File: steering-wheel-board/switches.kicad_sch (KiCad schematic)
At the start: 15 parts, among them SW2 SW_SPST, SW3 SW_SPST, SW4 SW_SPST

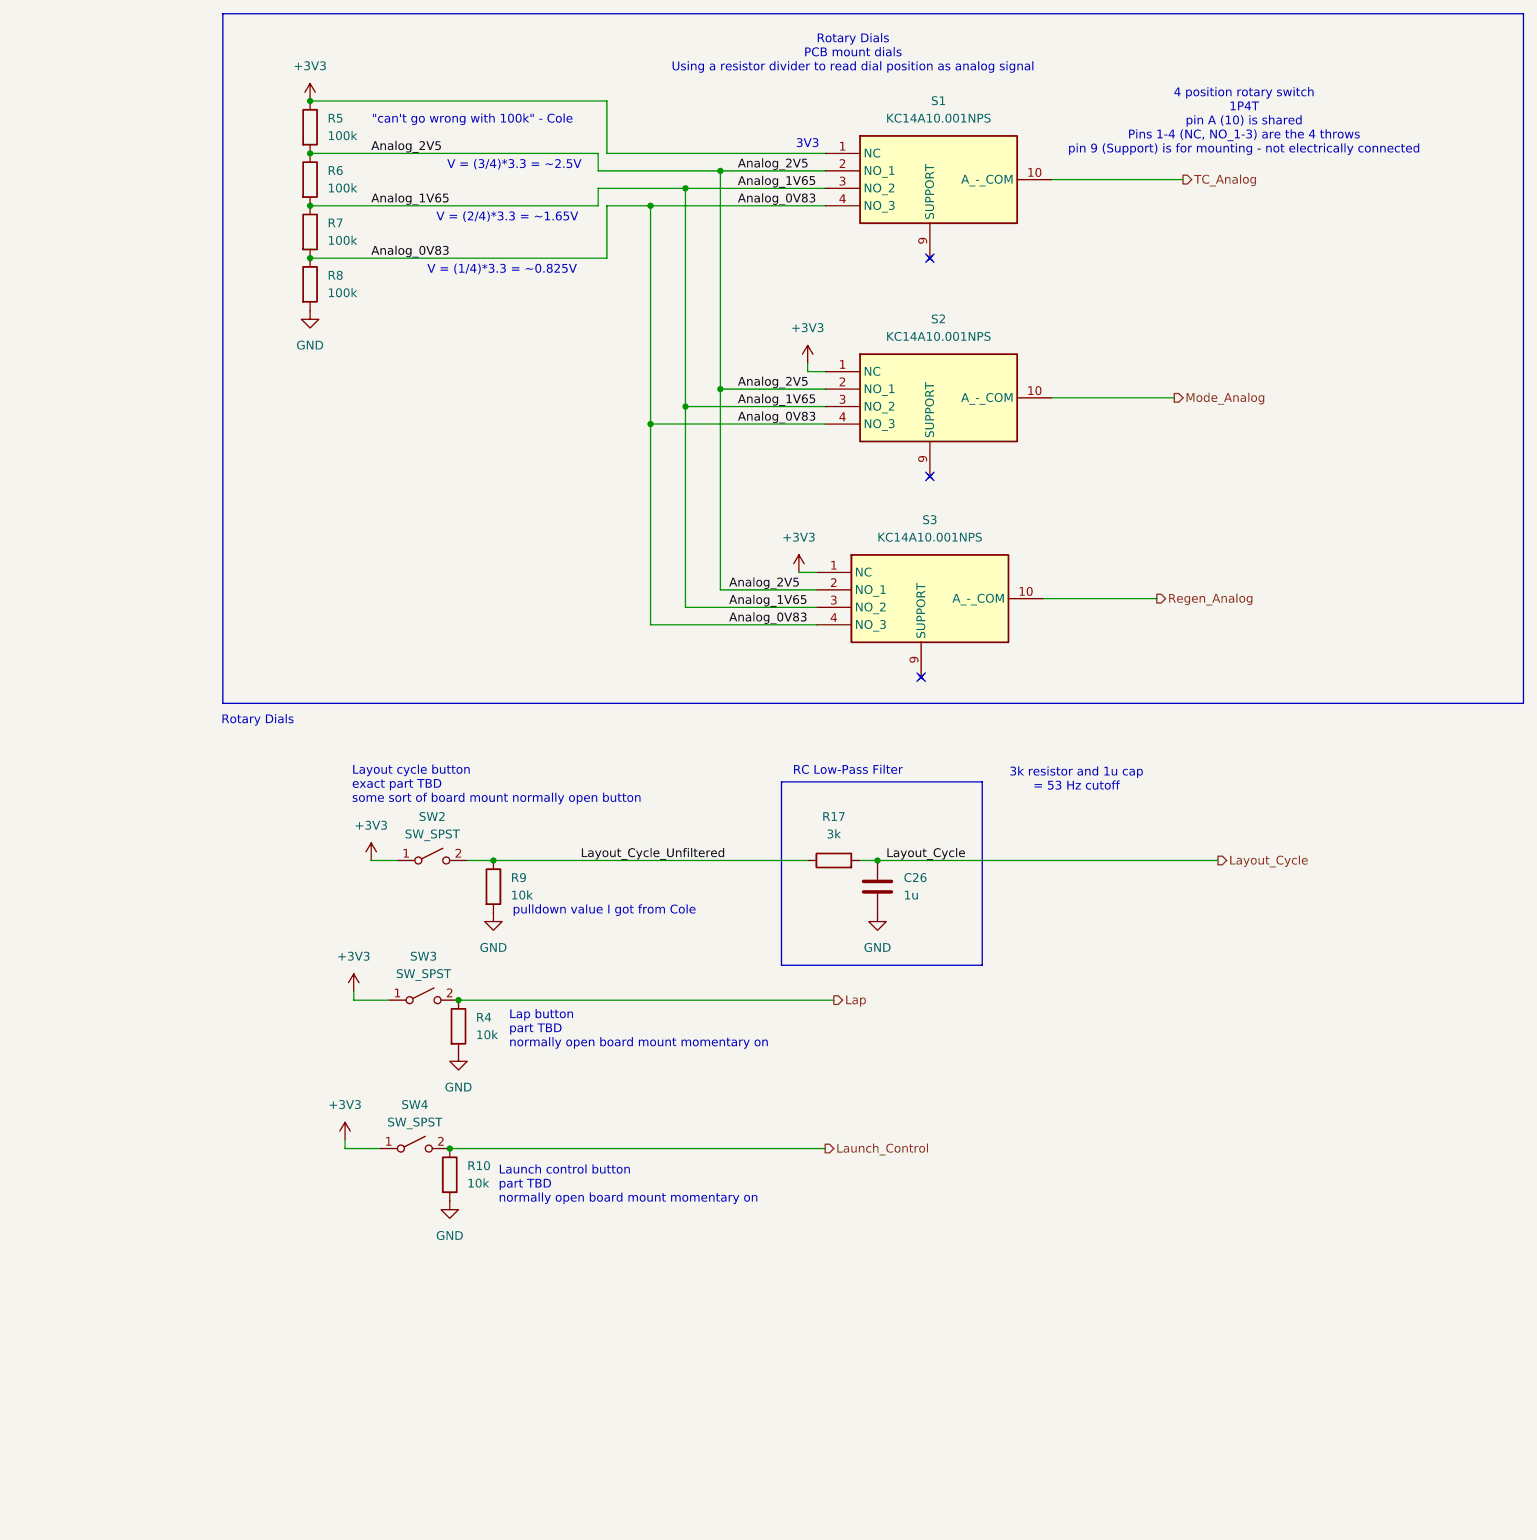
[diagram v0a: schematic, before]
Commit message: formatting changes, updated resistor ladder and CAN termination/aux can jumper
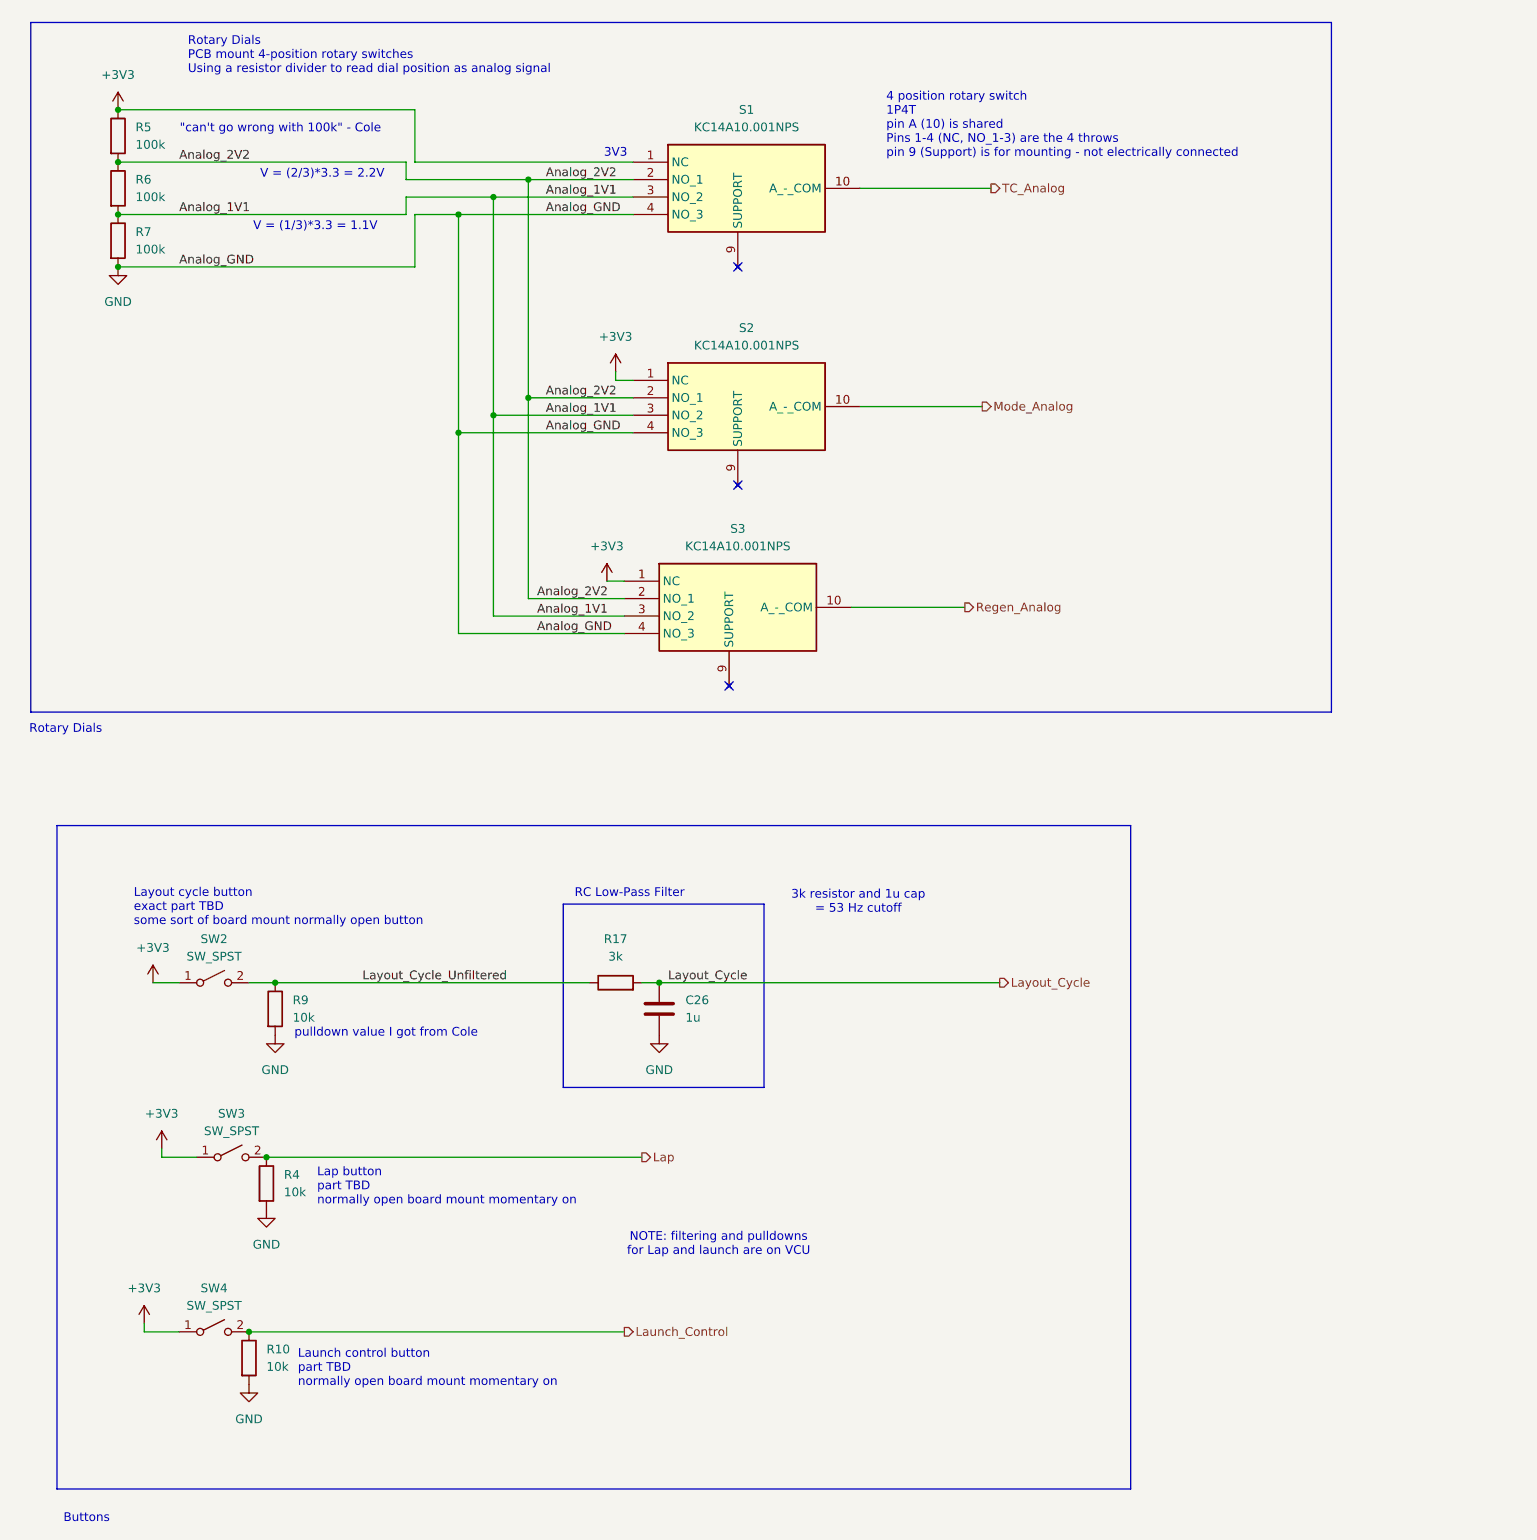
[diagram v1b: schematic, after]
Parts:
- removed R8: 100k, symbol Device:R
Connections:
- net Analog_0V83 is gone; now on net GND: R7.2, S1.4 (NO_3), S2.4 (NO_3), S3.4 (NO_3)
- net Analog_1V65 renamed Analog_1V1
- net Analog_2V5 renamed Analog_2V2
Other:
- note added: "Buttons"
- note added: "NOTE: filtering and pulldowns for Lap and launch are on VCU"
- note added: "Rotary Dials PCB mount 4-position rotary switches Using a resistor divider to read dial position as analog signal"
- note added: "V = (1/3)*3.3 = 1.1V"
- note added: "V = (2/3)*3.3 = 2.2V"
- note removed: "Rotary Dials PCB mount dials Using a resistor divider to read dial position as analog signal"
- note removed: "V = (1/4)*3.3 = ~0.825V"
- note removed: "V = (2/4)*3.3 = ~1.65V"
- note removed: "V = (3/4)*3.3 = ~2.5V"
- moved on the sheet: C26, R10, R17, R4, R5, R6, R7, R9, S1, S2, S3, SW2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
